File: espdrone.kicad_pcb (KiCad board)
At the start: 6 copper layers, 60 x 60 mm, 503 parts, among them J10 Conn_01x04, J11 Conn_01x04, J12 Conn_01x04, J4 Conn_01x06, J5 Conn_Coaxial, J6 Conn_01x06, J7 Conn_01x06, J8 Conn_01x04, J9 Conn_01x04, Q1 NMOS, Q10 NMOS, Q11 NMOS, Q12 NMOS, Q13 NMOS, Q14 NMOS, Q15 NMOS, Q16 NMOS, Q17 NMOS, Q18 NMOS, Q19 NMOS, Q2 NMOS, Q20 NMOS, Q21 NMOS, Q22 NMOS, Q23 NMOS, Q24 NMOS, Q25 NMOS, Q26 NMOS, Q27 NMOS, Q28 NMOS, Q3 NMOS, Q4 NMOS, Q5 NMOS, Q6 NMOS, Q7 NMOS, Q8 NMOS, Q9 NMOS, U10 FPC-1.0FX-15PWCR-H20, U11 VL53L1CXV0FY1, U12 LIS2MDL, U13 LSM6DS3, U14 PMW3901MB-TXQT_C43496881, U15 STM32G071K8U6, U16 DRV8328ARUYR, U18 STM32G071K8U6, U19 DRV8328ARUYR, U2 USBLC6-2P6, U20 INA180A2, U21 STM32G071K8U6, U22 DRV8328ARUYR, U23 INA180A2, U24 STM32G071K8U6, U25 DRV8328ARUYR, U26 INA180A2, U27 INA190A3IDCKR, U28 INA190A3IDCKR, U29 INA190A3IDCKR, U3 W25Q128JVP, U4 ESP32-C5HF4, U5 LFD182G45DCHD277, U6 TLV62569DBV, U7 INA190A3IDCKR, U8 TPS63070RNMR, U9 TPS2121RUXR, Y1 Crystal_GND24, Y2 Crystal_GND24

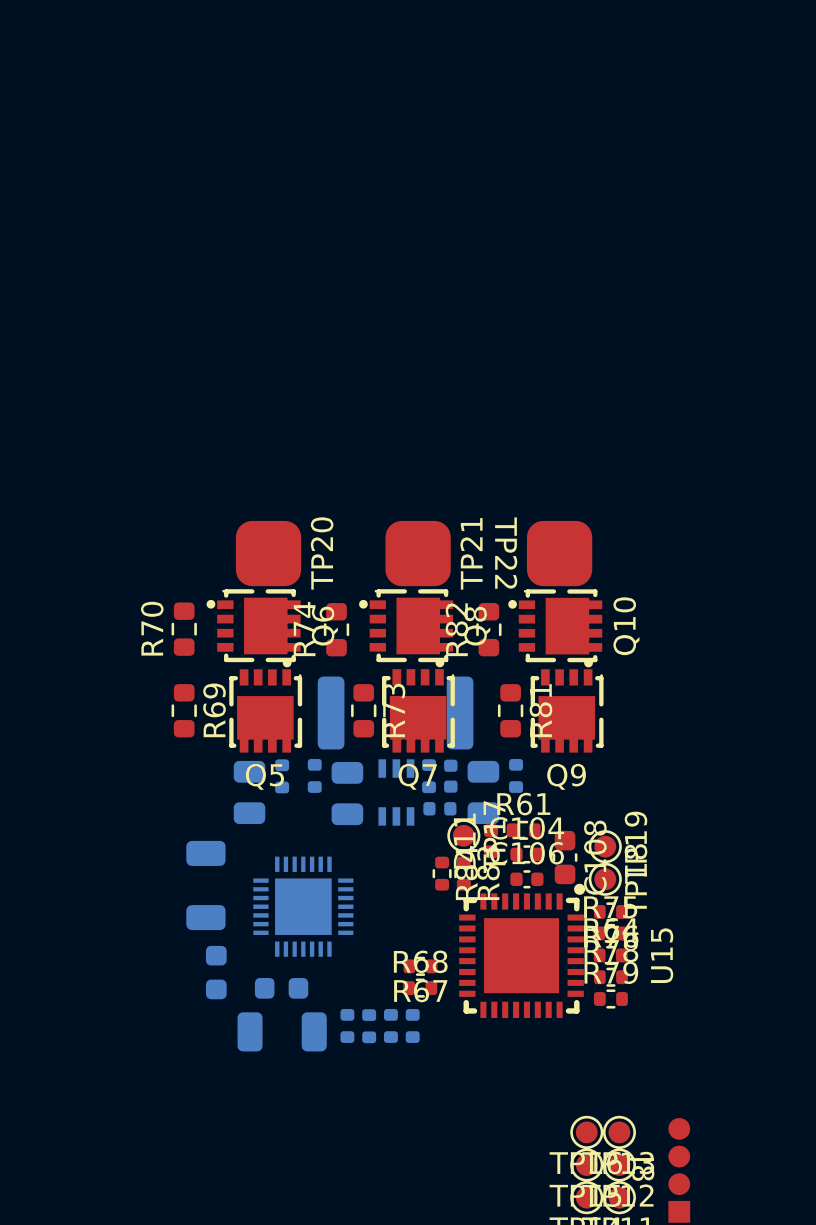
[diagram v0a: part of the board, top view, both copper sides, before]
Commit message: Progress on bridge layout
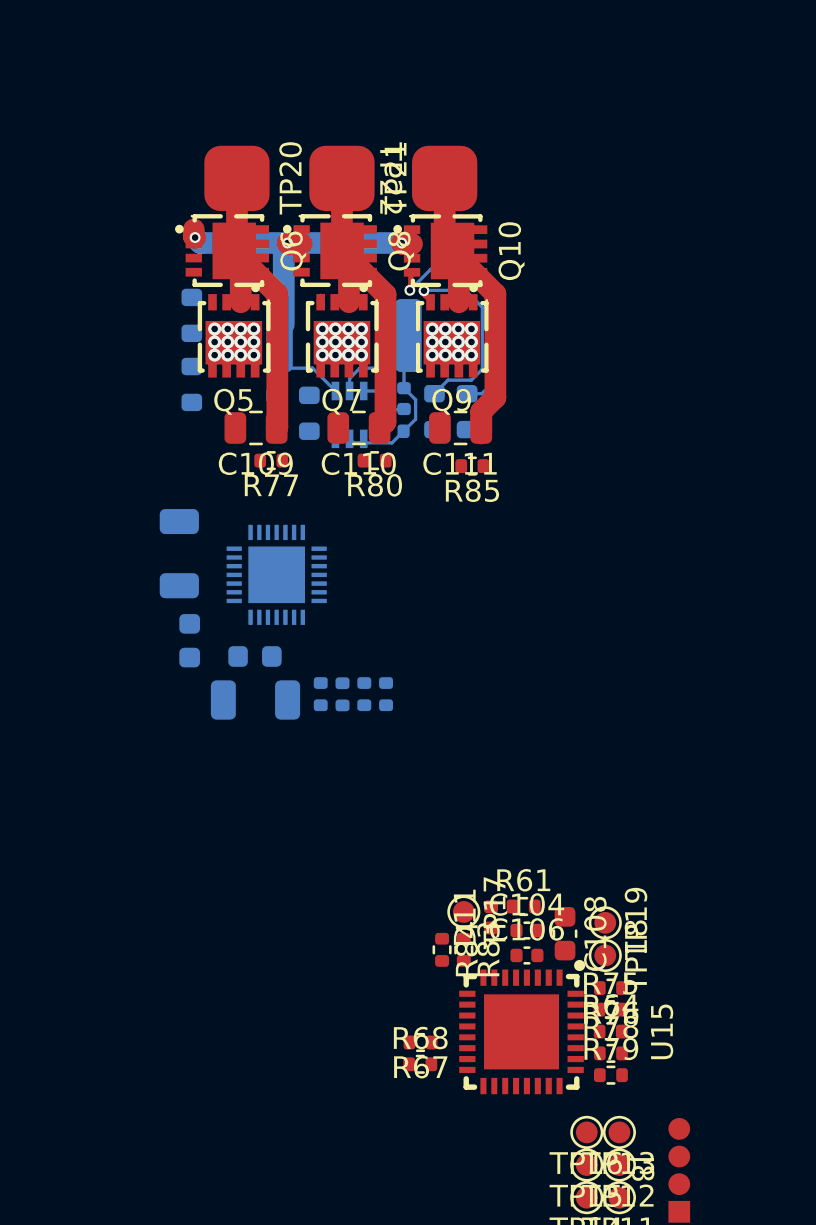
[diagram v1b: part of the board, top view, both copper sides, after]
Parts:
- C109, C110, C111, R77, R80, R85: moved to F.Cu
- R69, R70, R73, R74, R81, R82: moved to B.Cu
- moved Q10 18.0 mm to (129.5, 61.9)
- moved Q9 18.0 mm to (129.8, 65.8)
- moved TP22 18.0 mm to (126.5, 58.6)
- moved Q7 17.6 mm to (124.8, 65.8)
- moved Q8 17.6 mm to (124.4, 61.9)
- moved TP21 17.6 mm to (127.8, 58.5)
- moved R71 17.5 mm to (124.8, 65.8)
- moved C117 17.5 mm to (127.1, 70.2)
- moved C119 17.5 mm to (127.6, 68.7)
- moved R72 17.5 mm to (126.6, 68.7)
- moved U7 17.5 mm to (125.1, 69.4)
- moved Q5 17.3 mm to (119.8, 65.8)
- moved TP20 17.3 mm to (122.9, 58.5)
- moved Q6 17.3 mm to (119.5, 61.9)
- moved C110 16.8 mm to (125.5, 70.0), turned to 180 degrees
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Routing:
- net /Motors/ESC1/LSS: track 0.00 -> 17.9 mm, vias 0 -> 3
- net /Motors/ESC1/PHASE_C: track 0.00 -> 15.4 mm
- net /Motors/ESC1/PHASE_B: track 0.00 -> 14.9 mm
- net /Motors/ESC1/PHASE_A: track 0.00 -> 14.8 mm
- net Net-(Q10-G): track 0.00 -> 11.7 mm, vias 0 -> 1
- net GND: track 0.00 -> 11.6 mm
- net Net-(Q9-G): track 0.00 -> 9.36 mm, vias 0 -> 1
- net /Motors/ESC1/ISENSE: track 0.00 -> 1.01 mm
- net Net-(U7-OUT): track 0.00 -> 0.92 mm
- net +BATT: track 0.00 -> 0.11 mm, vias 0 -> 36
